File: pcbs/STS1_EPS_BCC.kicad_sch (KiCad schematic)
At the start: 45 parts, among them Q1 SI7135DP-T1-GE3, U1 LTC4020EUHFPBF, U2 SI7272DP-T1-GE3, U3 SI7272DP-T1-GE3

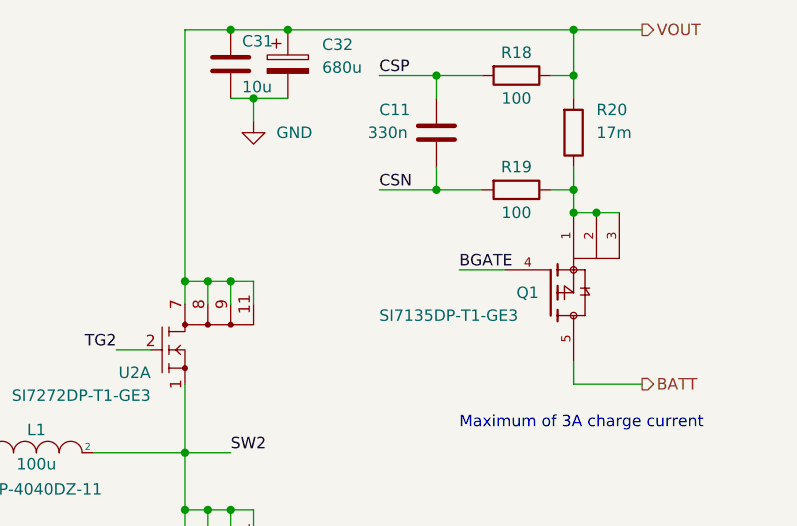
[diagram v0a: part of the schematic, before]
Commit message: Worked on STS1_EPS_1 layout.
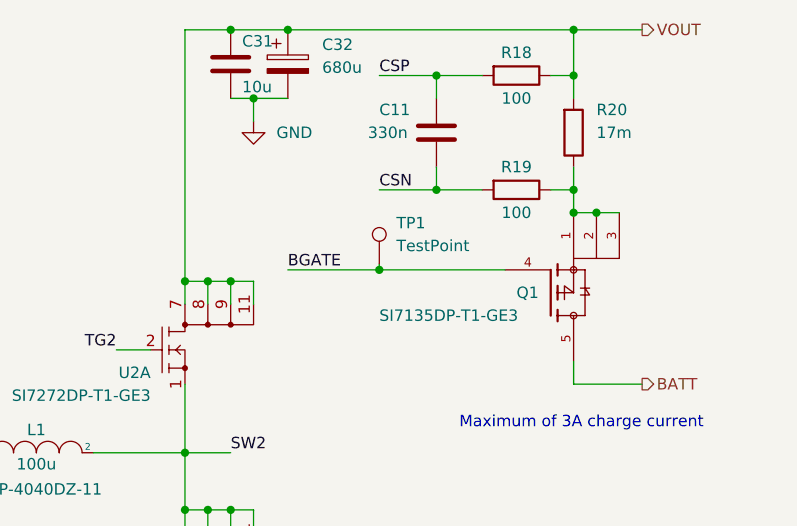
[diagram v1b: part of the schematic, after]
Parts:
- added TP1: TestPoint, Connector_Pin:Pin_D0.7mm_L6.5mm_W1.8mm_FlatFork, symbol Connector:TestPoint
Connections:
- net BGATE: now also TP1.1
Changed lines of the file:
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@@
   (junction (at 232.41 24.13) (diameter 0) (color 0 0 0 0)
   )
+  (junction (at 246.38 43.18) (diameter 0) (color 0 0 0 0)
+  )
   (junction (at 135.89 173.99) (diameter 0) (color 0 0 0 0)
   )
@@
     (stroke (width 0) (type default) (color 0 0 0 0))
   )
+  (wire (pts (xy 246.38 43.18) (xy 236.22 43.18))
+    (stroke (width 0) (type default) (color 0 0 0 0))
+  )
   (wire (pts (xy 232.41 69.85) (xy 232.41 72.39))
     (stroke (width 0) (type default) (color 0 0 0 0))
@@
     (stroke (width 0) (type default) (color 0 0 0 0))
   )
+  (wire (pts (xy 246.38 42.545) (xy 246.38 43.18))
+    (stroke (width 0) (type default) (color 0 0 0 0))
+  )
   (wire (pts (xy 52.07 100.33) (xy 52.07 102.87))
     (stroke (width 0) (type default) (color 0 0 0 0))
@@
     (stroke (width 0) (type default) (color 0 0 0 0))
   )
-  (wire (pts (xy 260.35 43.18) (xy 255.27 43.18))
+  (wire (pts (xy 246.38 43.18) (xy 260.35 43.18))
     (stroke (width 0) (type default) (color 0 0 0 0))
   )
@@
     (effects (font (size 1.27 1.27)) (justify left bottom))
   )
-  (label "BGATE" (at 255.27 43.18 0)
+  (label "BGATE" (at 236.22 43.18 0)
     (effects (font (size 1.27 1.27)) (justify left bottom))
   )
@@
     (pin "9")
   )
+  (symbol (lib_id "Connector:TestPoint") (at 246.38 42.545 0) (unit 1)
+    (in_bom yes) (on_board yes) (fields_autoplaced)
+    (property "Reference" "TP1" (id 0) (at 248.285 37.9729 0)
+      (effects (font (size 1.27 1.27)) (justify left))
+    )
+    (property "Value" "TestPoint" (id 1) (at 248.285 40.5129 0)
+      (effects (font (size 1.27 1.27)) (justify left))
+    )
+    (property "Footprint" "Connector_Pin:Pin_D0.7mm_L6.5mm_W1.8mm_FlatFork" (id 2) (at 251.46 42.545 0)
+      (effects (font (size 1.27 1.27)) hide)
+    )
+    (property "Datasheet" "~" (id 3) (at 251.46 42.545 0)
+      (effects (font (size 1.27 1.27)) hide)
+    )
+    (pin "1")
+  )
   (symbol (lib_id "power:GND") (at 74.93 59.69 270) (unit 1)
